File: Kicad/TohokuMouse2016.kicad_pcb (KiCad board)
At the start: 2 copper layers, 67.6 x 35 mm, 77 parts, among them P1 BATTERY_CON, P2 DOWNLOAD, P3 L_MOTOR, P4 R_MOTOR, P5 L_ENC_MAIN, P6 R_ENC_MAIN, P7 L_ENC_SUB, P8 R_ENC_SUB, Q1 LTR-4206E, Q2 RUM003N02, Q3 LTR-4206E, Q4 RUM003N02, Q5 LTR-4206E, Q6 LTR-4206E, Q7 RUM003N02, Q8 ZXM62P02E6, Q9 RUM003N02, SW1 MAIN_SW, SW2 PUSH_SW, U1 MPU-6500, U2 AP7333-28SRG-7, U3 AP7333-28SRG-7, U4 R5F5631MCDFL, U5 DRV8836, U6 AS5055, U7 AS5055, X1 CSTCE12M0G55-R0

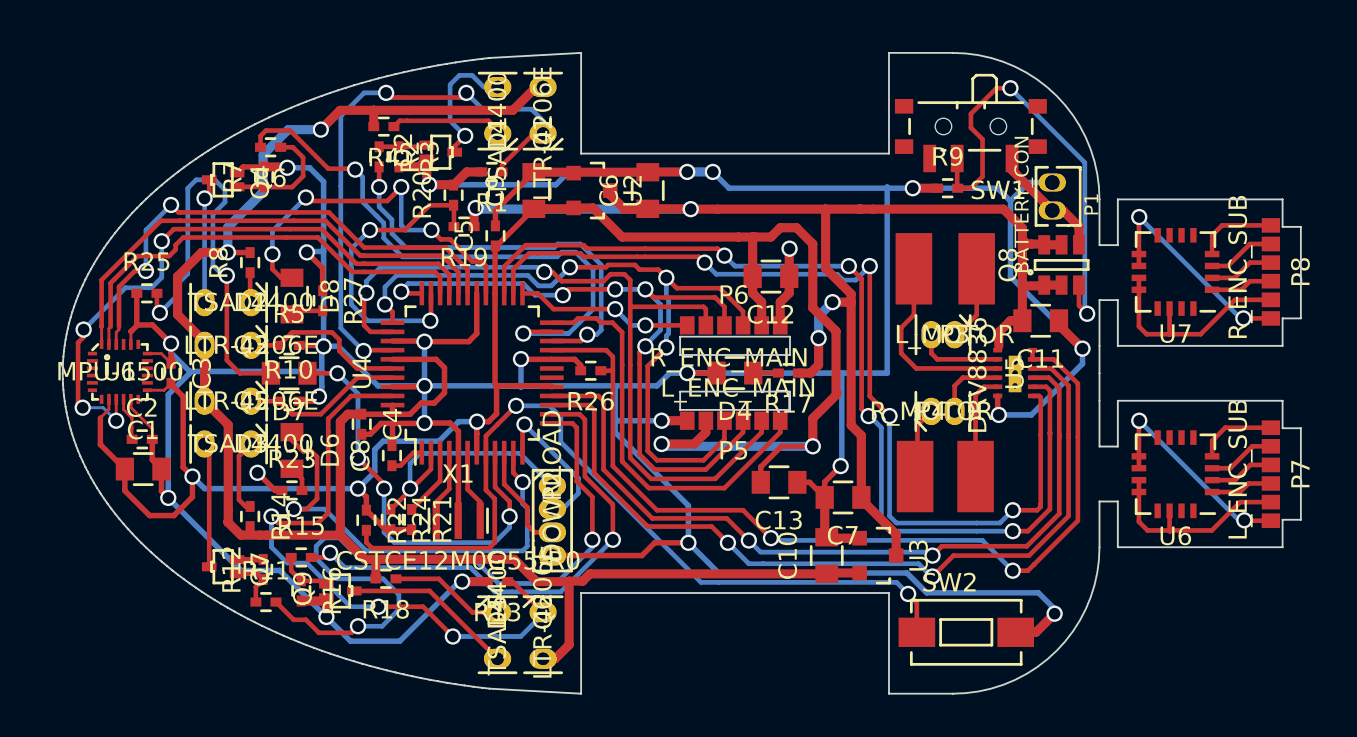
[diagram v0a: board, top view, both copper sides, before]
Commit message: fin
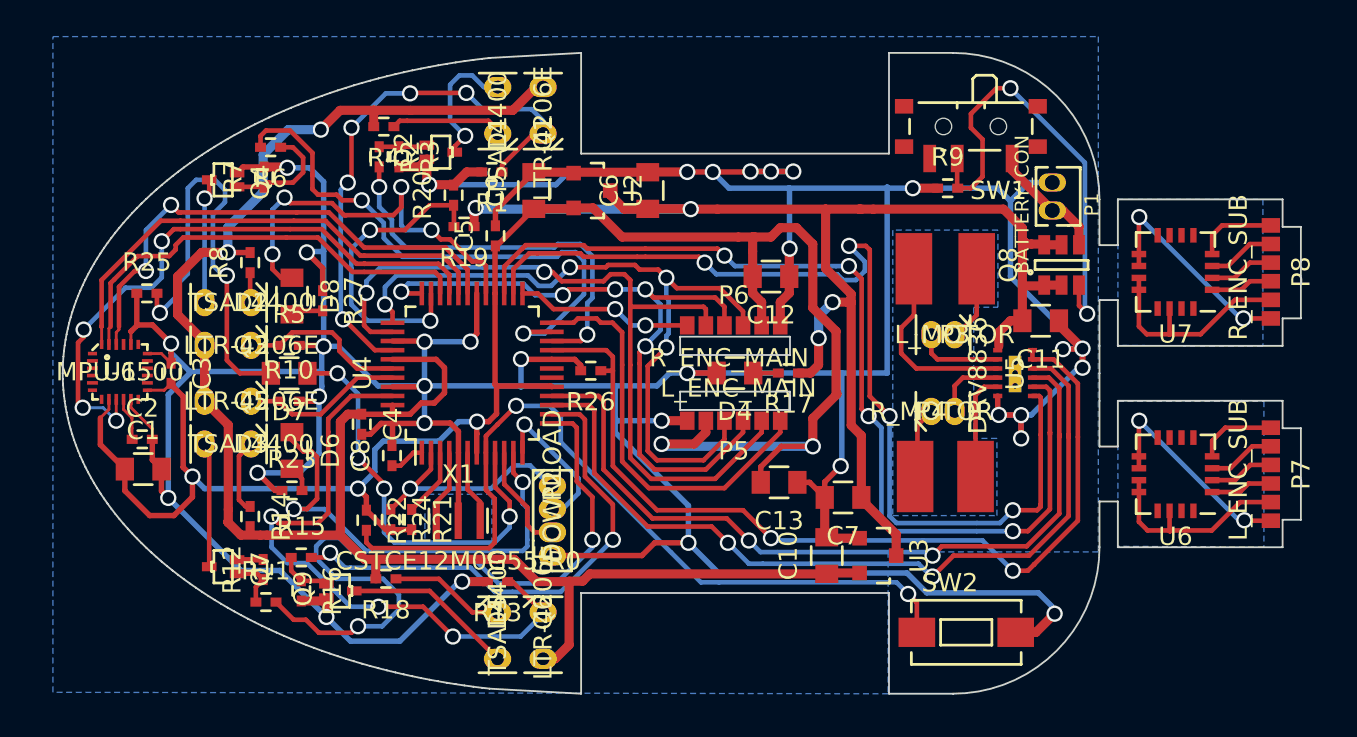
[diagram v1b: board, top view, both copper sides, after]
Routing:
- net GND: track 294.3 -> 319.5 mm, vias 25 -> 33
- net /R_PULSE: track 51.4 -> 54.9 mm
- net /LED2: track 20.7 -> 22.9 mm
- net /MD: track 14.2 -> 12.8 mm
- net /FR_AD: track 31.4 -> 30.1 mm, vias 3 -> 5
- net /RS_ON: track 31.7 -> 30.9 mm
- net /FR_ON: track 22.7 -> 22.0 mm
- added copper zone on B.Cu, net GND
- added copper zone on B.Cu, net Net-(P7-Pad6)
- added copper zone on B.Cu, net Net-(P8-Pad6)

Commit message: Order to elerow.
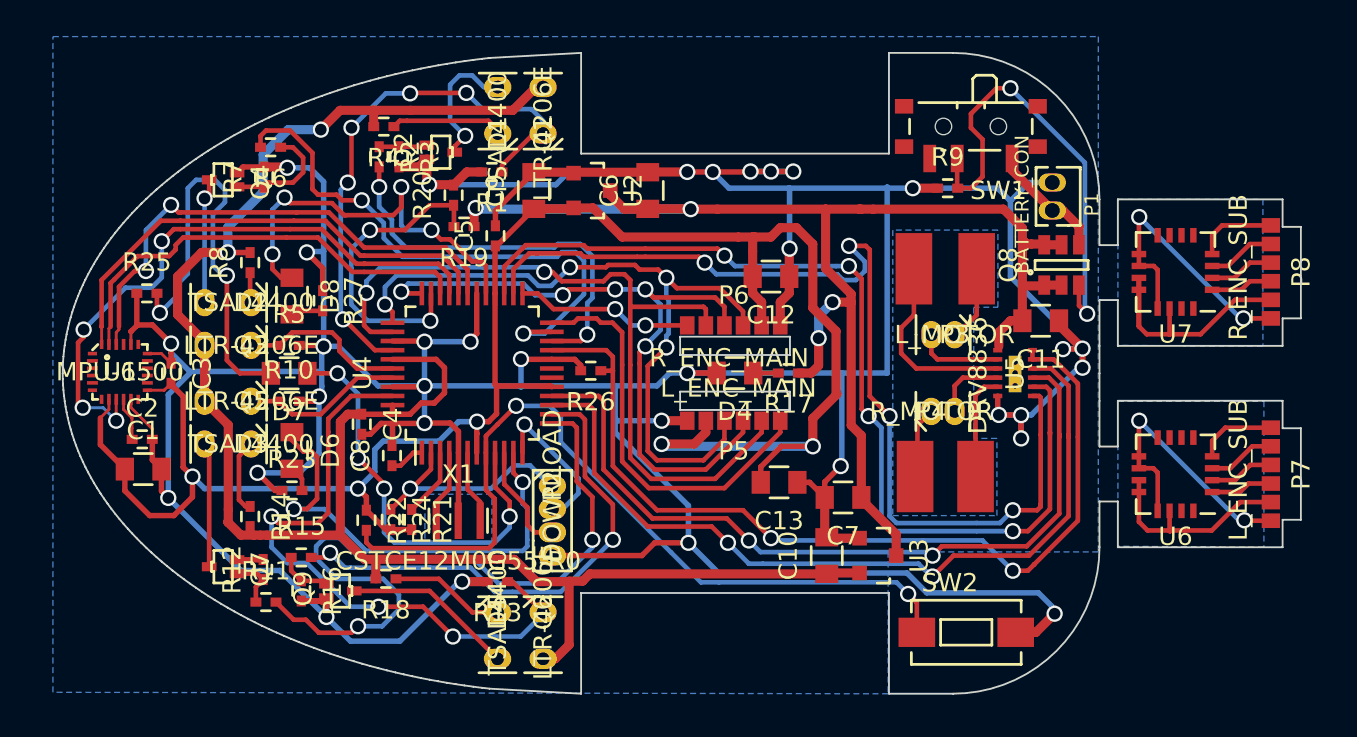
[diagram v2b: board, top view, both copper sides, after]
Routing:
- net GND: track 319.5 -> 323.1 mm
- net Net-(P8-Pad6): track 12.2 -> 15.4 mm
- net Net-(P7-Pad6): track 12.1 -> 15.3 mm
- net Net-(P8-Pad5): track 12.2 -> 14.9 mm
- net VCC: track 108.9 -> 111.1 mm
- net VEE: track 103.3 -> 103.8 mm
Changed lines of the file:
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@@
   (general
     (links 186)
-    (no_connects 8)
-    (area 99.949999 64.949999 167.680001 100.050001)
+    (no_connects 3)
+    (area 95.657999 62.383999 176.249001 102.335001)
     (thickness 1.6)
     (drawings 242)
-    (tracks 1244)
+    (tracks 1265)
     (zones 0)
     (modules 77)
@@
   (layers
     (0 F.Cu signal)
-    (31 B.Cu signal)
+    (31 B.Cu signal hide)
     (32 B.Adhes user)
     (33 F.Adhes user)
@@
     (visible_elements 7FFCF7FF)
     (pcbplotparams
-      (layerselection 0x00030_80000001)
+      (layerselection 0x010e0_80000001)
       (usegerberextensions true)
       (excludeedgelayer true)
@@
       (psa4output false)
       (plotreference true)
-      (plotvalue true)
+      (plotvalue false)
       (plotinvisibletext false)
       (padsonsilk false)
-      (subtractmaskfromsilk false)
+      (subtractmaskfromsilk true)
       (outputformat 1)
       (mirror false)
-      (drillshape 1)
+      (drillshape 0)
       (scaleselection 1)
-      (outputdirectory ""))
+      (outputdirectory product_data/))
   )
   (net 0 "")
@@
   (gr_line (start 136.779 82.4865) (end 176.149 82.4865) (angle 90) (layer Cmts.User) (width 0.2))
   (segment (start 137.7155 82.4865) (end 139.0865 82.4865) (width 0.254) (layer F.Cu) (net 1))
+  (segment (start 114.4016 95.8088) (end 114.4016 94.7674) (width 0.3) (layer F.Cu) (net 2))
+  (segment (start 114.4016 94.7674) (end 114.2326 94.9364) (width 0.3) (layer F.Cu) (net 2))
+  (segment (start 114.2326 94.9364) (end 113.03 94.9364) (width 0.3) (layer F.Cu) (net 2))
+  (segment (start 113.03 94.9364) (end 114.2326 94.9364) (width 0.3) (layer F.Cu) (net 2))
+  (segment (start 114.2326 94.9364) (end 114.4016 95.1054) (width 0.3) (layer F.Cu) (net 2))
+  (segment (start 114.4016 95.1054) (end 114.4016 95.8088) (width 0.3) (layer F.Cu) (net 2))
+  (segment (start 114.2326 94.9364) (end 114.4016 95.1054) (width 0.3) (layer F.Cu) (net 2))
+  (segment (start 114.4016 95.1054) (end 114.4016 95.8088) (width 0.3) (layer F.Cu) (net 2))
+  (segment (start 114.2326 94.9364) (end 114.4016 94.7674) (width 0.3) (layer F.Cu) (net 2))
   (segment (start 135.509 71.501) (end 137.541 71.501) (width 0.3) (layer F.Cu) (net 2))
   (segment (start 137.541 71.501) (end 137.5664 71.4756) (width 0.3) (layer F.Cu) (net 2))
@@
   (segment (start 121.666 93.8784) (end 118.4148 97.1296) (width 0.3) (layer B.Cu) (net 2))
   (via (at 114.4016 95.8088) (size 0.889) (drill 0.635) (layers F.Cu B.Cu) (net 2))
-  (segment (start 114.4016 95.8088) (end 114.4016 94.7674) (width 0.5) (layer F.Cu) (net 2))
-  (segment (start 113.03 94.9364) (end 114.2326 94.9364) (width 0.5) (layer F.Cu) (net 2))
   (segment (start 114.2326 94.9364) (end 114.4016 94.7674) (width 0.5) (layer F.Cu) (net 2))
   (segment (start 119.888 70.8025) (end 119.888 72.0725) (width 0.5) (layer F.Cu) (net 2))
@@
   (segment (start 133.096 80.3275) (end 133.096 78.486) (width 0.254) (layer B.Cu) (net 10))
   (segment (start 132.969 80.4545) (end 133.096 80.3275) (width 0.254) (layer B.Cu) (net 10))
+  (segment (start 137.7188 75.057) (end 137.7188 77.1812) (width 0.3) (layer F.Cu) (net 11))
+  (segment (start 137.7188 77.1812) (end 137.684 77.216) (width 0.3) (layer F.Cu) (net 11))
   (segment (start 117.9068 86.2076) (end 117.5004 86.2076) (width 0.3) (layer B.Cu) (net 11))
   (segment (start 121.6152 85.1408) (end 120.5484 86.2076) (width 0.3) (layer B.Cu) (net 11))
@@
   (segment (start 122.6145 85.1575) (end 122.6145 85.8012) (width 0.3) (layer F.Cu) (net 11))
   (segment (start 140.97 77.1525) (end 140.97 78.9305) (width 0.5) (layer F.Cu) (net 11))
-  (segment (start 137.684 75.057) (end 138.684 75.057) (width 0.5) (layer F.Cu) (net 11))
+  (segment (start 137.684 75.057) (end 137.7188 75.057) (width 0.5) (layer F.Cu) (net 11))
+  (segment (start 137.7188 75.057) (end 138.684 75.057) (width 0.5) (layer F.Cu) (net 11))
   (segment (start 140.081 74.549) (end 140.97 75.438) (width 0.5) (layer F.Cu) (net 11))
   (segment (start 139.192 74.549) (end 140.081 74.549) (width 0.5) (layer F.Cu) (net 11))
@@
   (segment (start 164.3028 88.986) (end 162.782 88.986) (width 0.254) (layer F.Cu) (net 17))
   (segment (start 164.7698 88.519) (end 164.3028 88.986) (width 0.254) (layer F.Cu) (net 17))
+  (segment (start 159.807 90.011) (end 159.807 87.925) (width 0.254) (layer F.Cu) (net 18))
+  (segment (start 159.568 87.686) (end 158.782 87.686) (width 0.254) (layer F.Cu) (net 18))
+  (segment (start 159.807 87.925) (end 159.568 87.686) (width 0.254) (layer F.Cu) (net 18))
   (segment (start 158.782 87.036) (end 158.782 85.1088) (width 0.254) (layer F.Cu) (net 18))
   (segment (start 164.5666 90.551) (end 164.5412 90.5256) (width 0.254) (layer F.Cu) (net 18))
@@
   (segment (start 164.0384 88.336) (end 162.782 88.336) (width 0.254) (layer F.Cu) (net 21))
   (segment (start 164.8714 87.503) (end 164.0384 88.336) (width 0.254) (layer F.Cu) (net 21))
+  (segment (start 158.782 77.287) (end 158.782 77.937) (width 0.254) (layer F.Cu) (net 22))
+  (segment (start 158.782 77.937) (end 158.782 79.9404) (width 0.254) (layer F.Cu) (net 22))
   (segment (start 160.457 78.962) (end 160.457 80.3656) (width 0.254) (layer F.Cu) (net 22))
   (segment (start 160.457 80.3656) (end 160.4264 80.3656) (width 0.254) (layer F.Cu) (net 22))
@@
   (segment (start 164.379 77.937) (end 162.782 77.937) (width 0.254) (layer F.Cu) (net 23))
   (segment (start 164.846 77.47) (end 164.379 77.937) (width 0.254) (layer F.Cu) (net 23))
+  (segment (start 159.807 78.962) (end 159.807 76.8506) (width 0.254) (layer F.Cu) (net 24))
+  (segment (start 159.5934 76.637) (end 158.782 76.637) (width 0.254) (layer F.Cu) (net 24))
+  (segment (start 159.807 76.8506) (end 159.5934 76.637) (width 0.254) (layer F.Cu) (net 24))
   (segment (start 158.782 75.987) (end 158.782 73.9836) (width 0.254) (layer F.Cu) (net 24))
   (via (at 164.4904 79.502) (size 0.889) (drill 0.635) (layers F.Cu B.Cu) (net 24))
@@
   (segment (start 125.73 69.4055) (end 123.994 71.1415) (width 0.254) (layer F.Cu) (net 28))
   (segment (start 123.994 71.1415) (end 123.994 71.501) (width 0.254) (layer F.Cu) (net 28))
+  (segment (start 110.236 90.8724) (end 110.236 91.1352) (width 0.3) (layer F.Cu) (net 29))
+  (segment (start 110.236 91.1352) (end 110.4392 91.3384) (width 0.3) (layer F.Cu) (net 29))
   (segment (start 115.5739 84.7305) (end 116.332 84.7305) (width 0.5) (layer F.Cu) (net 29))
   (segment (start 115.1636 85.1408) (end 115.5739 84.7305) (width 0.5) (layer F.Cu) (net 29))
@@
   (segment (start 109.0422 90.6526) (end 109.0168 90.6272) (width 0.5) (layer F.Cu) (net 29))
   (segment (start 111.1504 91.3384) (end 110.7948 91.3384) (width 0.5) (layer F.Cu) (net 29))
-  (segment (start 110.7948 91.3384) (end 109.728 91.3384) (width 0.5) (layer F.Cu) (net 29))
+  (segment (start 110.7948 91.3384) (end 110.4392 91.3384) (width 0.5) (layer F.Cu) (net 29))
+  (segment (start 110.4392 91.3384) (end 109.728 91.3384) (width 0.5) (layer F.Cu) (net 29))
   (segment (start 111.1504 91.3384) (end 115.1636 91.3384) (width 0.5) (layer F.Cu) (net 29))
   (segment (start 109.728 91.3384) (end 109.0168 90.6272) (width 0.5) (layer F.Cu) (net 29))
@@
   (segment (start 124.2988 93.8784) (end 124.5616 93.8784) (width 0.254) (layer F.Cu) (net 32))
   (segment (start 124.5616 93.8784) (end 126.238 95.5548) (width 0.254) (layer F.Cu) (net 32))
+  (segment (start 140.1865 82.4865) (end 140.8811 82.4865) (width 0.5) (layer F.Cu) (net 33))
+  (via (at 141.2875 80.5815) (size 0.889) (drill 0.635) (layers F.Cu B.Cu) (net 33))
+  (segment (start 142.0495 78.613) (end 143.0655 78.613) (width 0.5) (layer F.Cu) (net 33))
+  (via (at 142.0495 78.613) (size 0.889) (drill 0.635) (layers F.Cu B.Cu) (net 33))
+  (segment (start 141.2875 79.375) (end 142.0495 78.613) (width 0.5) (layer B.Cu) (net 33))
+  (segment (start 141.2875 80.5815) (end 141.2875 79.375) (width 0.5) (layer B.Cu) (net 33))
+  (segment (start 141.2875 82.0801) (end 141.2875 80.5815) (width 0.5) (layer F.Cu) (net 33))
+  (segment (start 140.8811 82.4865) (end 141.2875 82.0801) (width 0.5) (layer F.Cu) (net 33))
   (segment (start 122.47 74.4855) (end 122.47 73.5545) (width 0.5) (layer F.Cu) (net 33))
   (segment (start 122.6185 73.533) (end 122.555 73.4695) (width 0.5) (layer B.Cu) (net 33))
@@
   (segment (start 134.3025 73.533) (end 135.763 73.533) (width 0.5) (layer F.Cu) (net 33))
   (segment (start 134.2865 73.517) (end 134.3025 73.533) (width 0.5) (layer F.Cu) (net 33))
-  (segment (start 141.2875 80.5815) (end 141.2875 79.375) (width 0.5) (layer B.Cu) (net 33))
-  (segment (start 140.843 82.4865) (end 141.2875 82.042) (width 0.5) (layer F.Cu) (net 33))
-  (segment (start 141.2875 82.042) (end 141.2875 80.5815) (width 0.5) (layer F.Cu) (net 33))
-  (via (at 141.2875 80.5815) (size 0.889) (drill 0.635) (layers F.Cu B.Cu) (net 33))
-  (segment (start 140.1865 82.4865) (end 140.843 82.4865) (width 0.5) (layer F.Cu) (net 33))
-  (segment (start 142.0495 78.613) (end 143.0655 78.613) (width 0.5) (layer F.Cu) (net 33))
-  (via (at 142.0495 78.613) (size 0.889) (drill 0.635) (layers F.Cu B.Cu) (net 33))
-  (segment (start 141.2875 79.375) (end 142.0495 78.613) (width 0.5) (layer B.Cu) (net 33))
   (segment (start 143.0655 78.613) (end 142.875 78.613) (width 0.5) (layer F.Cu) (net 33))
   (segment (start 142.875 78.613) (end 143.0655 78.613) (width 0.5) (layer F.Cu) (net 33))
